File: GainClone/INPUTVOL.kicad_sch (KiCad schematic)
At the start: 25 parts, among them J4 AUDIO IN, U2 OPA1656ID, U7 CS3310

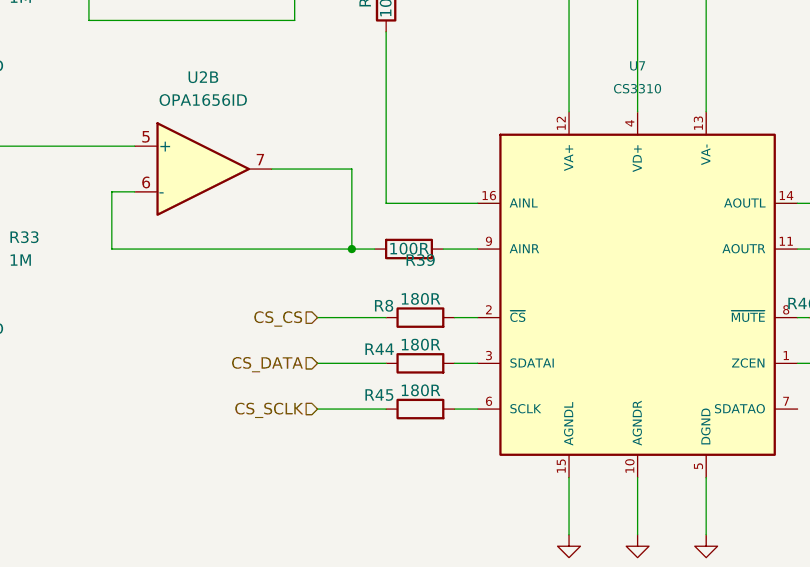
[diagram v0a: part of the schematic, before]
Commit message: commit
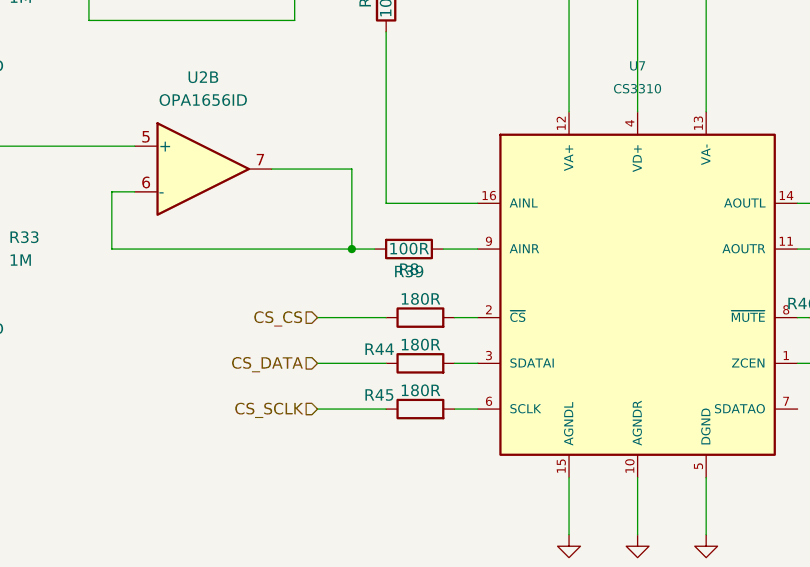
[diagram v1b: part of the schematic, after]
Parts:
- R7, R8: footprint Resistor_THT:R_Axial_DIN0207_L6.3mm_D2.5mm_P10.16mm_Horizontal -> Resistor_SMD:R_0805_2012Metric_Pad1.20x1.40mm_HandSolder
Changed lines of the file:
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@@
 			)
 		)
-		(property "Footprint" "Resistor_THT:R_Axial_DIN0207_L6.3mm_D2.5mm_P10.16mm_Horizontal"
+		(property "Footprint" "Resistor_SMD:R_0805_2012Metric_Pad1.20x1.40mm_HandSolder"
 			(at 137.668 78.74 90)
 			(hide yes)
@@
 	(symbol
 		(lib_id "Device:R")
-		(at 138.43 106.68 270)
-		(unit 1)
-		(body_style 1)
-		(exclude_from_sim no)
-		(in_bom yes)
-		(on_board yes)
-		(in_pos_files yes)
-		(dnp no)
-		(property "Reference" "R8"
-			(at 135.636 113.03 90)
-			(show_name no)
-			(do_not_autoplace no)
-			(effects
-				(font
-					(size 1.27 1.27)
-				)
-			)
-		)
-		(property "Value" "100R"
-			(at 138.43 106.68 90)
-			(show_name no)
-			(do_not_autoplace no)
-			(effects
-				(font
-					(size 1.27 1.27)
-				)
-			)
-		)
-		(property "Footprint" "Resistor_THT:R_Axial_DIN0207_L6.3mm_D2.5mm_P10.16mm_Horizontal"
-			(at 138.43 104.902 90)
-			(hide yes)
-			(show_name no)
-			(do_not_autoplace no)
-			(effects
-				(font
-					(size 1.27 1.27)
-				)
-			)
-		)
-		(property "Datasheet" ""
-			(at 138.43 106.68 0)
-			(hide yes)
-			(show_name no)
-			(do_not_autoplace no)
-			(effects
-				(font
-					(size 1.27 1.27)
-				)
-			)
-		)
-		(property "Description" "Resistor"
-			(at 138.43 106.68 0)
-			(hide yes)
-			(show_name no)
-			(do_not_autoplace no)
-			(effects
-				(font
-					(size 1.27 1.27)
-				)
-			)
-		)
-		(pin "1"
-		)
-		(pin "2"
-		)
-		(instances
-			(project "GainClone"
-				(path "/08655295-5783-460d-a904-560b6403a812/67b44205-e610-4be0-b03a-495a138c24e6"
-					(reference "R8")
-					(unit 1)
-				)
-			)
-		)
-	)
-	(symbol
-		(lib_id "Device:R")
 		(at 87.63 95.25 90)
 		(unit 1)
@@
 		(dnp no)
 		(property "Reference" "R39"
-			(at 139.7 107.95 90)
+			(at 138.43 109.22 90)
 			(show_name no)
 			(do_not_autoplace no)
@@
 					(unit 1)
 				)
+			)
+		)
+	)
+	(symbol
+		(lib_id "Device:R")
+		(at 138.43 106.68 270)
+		(unit 1)
+		(body_style 1)
+		(exclude_from_sim no)
+		(in_bom yes)
+		(on_board yes)
+		(in_pos_files yes)
+		(dnp no)
+		(property "Reference" "R8"
+			(at 138.43 108.966 90)
+			(show_name no)
+			(do_not_autoplace no)
+			(effects
+				(font
+					(size 1.27 1.27)
+				)
+			)
+		)
+		(property "Value" "100R"
+			(at 138.43 106.68 90)
+			(show_name no)
+			(do_not_autoplace no)
+			(effects
+				(font
+					(size 1.27 1.27)
+				)
+			)
+		)
+		(property "Footprint" "Resistor_SMD:R_0805_2012Metric_Pad1.20x1.40mm_HandSolder"
+			(at 138.43 104.902 90)
+			(hide yes)
+			(show_name no)
+			(do_not_autoplace no)
+			(effects
+				(font
+					(size 1.27 1.27)
+				)
+			)
+		)
+		(property "Datasheet" ""
+			(at 138.43 106.68 0)
+			(hide yes)
+			(show_name no)
+			(do_not_autoplace no)
+			(effects
+				(font
+					(size 1.27 1.27)
+				)
+			)
+		)
+		(property "Description" "Resistor"
+			(at 138.43 106.68 0)
+			(hide yes)
+			(show_name no)
+			(do_not_autoplace no)
+			(effects
+				(font
+					(size 1.27 1.27)
+				)
+			)
+		)
+		(pin "1"
+		)
+		(pin "2"
+		)
+		(instances
+			(project "GainClone"
+				(path "/08655295-5783-460d-a904-560b6403a812/67b44205-e610-4be0-b03a-495a138c24e6"
+					(reference "R8")
+					(unit 1)
+				)
